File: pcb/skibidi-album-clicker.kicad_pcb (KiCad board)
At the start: 2 copper layers, 28 x 60 mm, 28 parts, among them J1 Conn_01x02_Socket, Q1 Q_PMOS_GSD, Q2 Q_NMOS_GSD, SW1 RotaryEncoder_Switch, U1 XIAO-RP2040-DIP, U2 MCP73831-2-OT

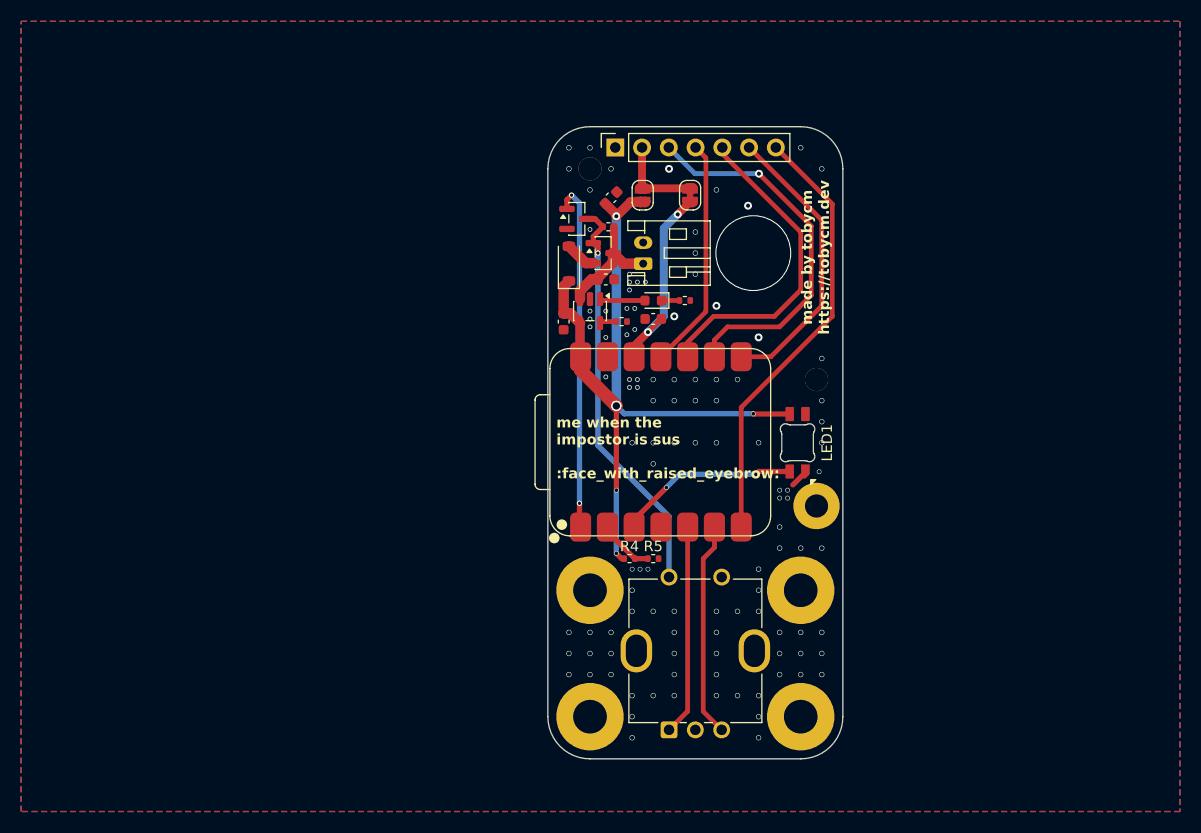
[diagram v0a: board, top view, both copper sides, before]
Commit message: update
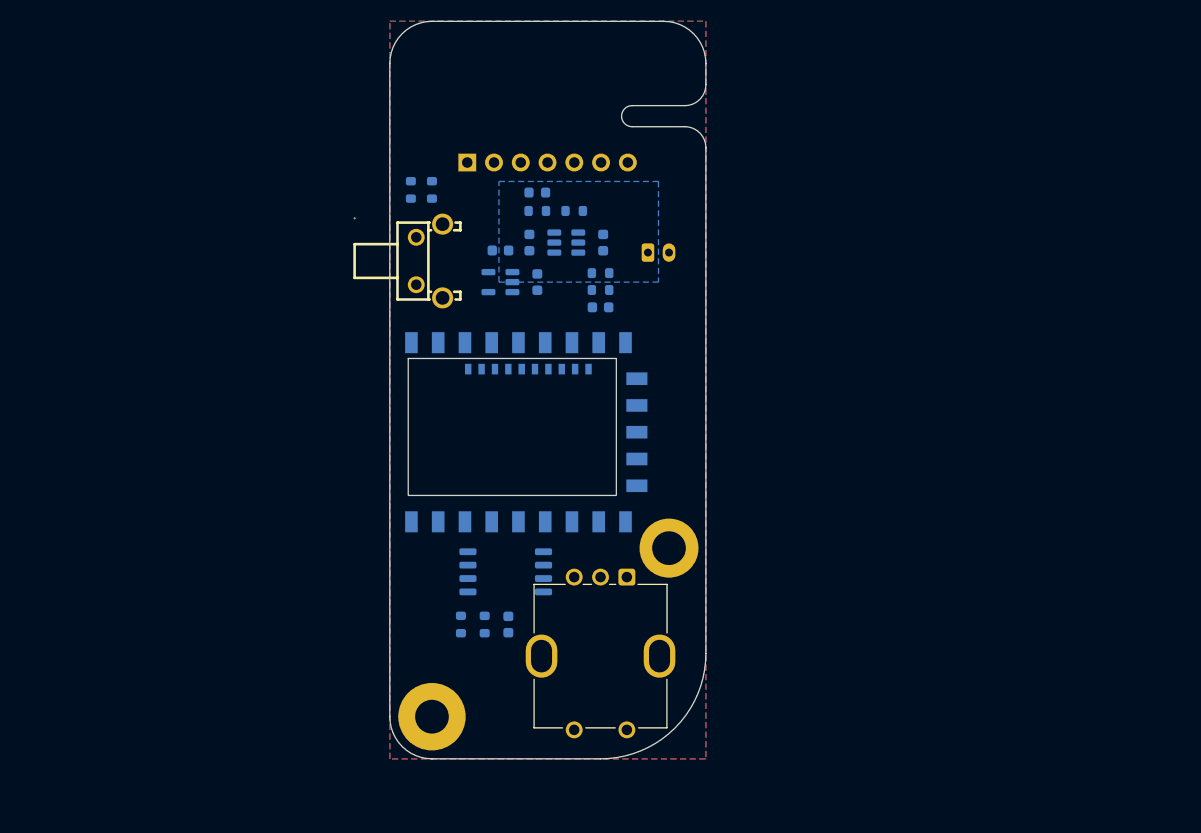
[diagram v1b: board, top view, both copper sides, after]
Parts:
- removed C2, C3: 4.7u, Capacitor_SMD:C_0603_1608Metric
- removed D2: D_Schottky, Diode_SMD:D_SOD-123
- removed H3, H4: MountingHole, MountingHole:MountingHole_3.2mm_M3_Pad
- removed H5, H7, H8: MountingHole, MountingHole:MountingHole_2.2mm_M2_Pad
- removed JP1: SolderJumper_2_Bridged, Jumper:SolderJumper-2_P1.3mm_Bridged_RoundedPad1.0x1.5mm
- removed JP2: SolderJumper_2_Open, Jumper:SolderJumper-2_P1.3mm_Open_RoundedPad1.0x1.5mm
- removed LED1: SK6812MINI-E, PCM_marbastlib-various:LED_6028R
- removed Q1: Q_PMOS_GSD, Package_TO_SOT_SMD:SOT-23
- removed Q2: Q_NMOS_GSD, Package_TO_SOT_SMD:SOT-23
- added C5: 10u, Capacitor_SMD:C_0603_1608Metric, B.Cu at (198.2, 71.0)
- added C6: 10u, Capacitor_SMD:C_0603_1608Metric, B.Cu at (205.2, 71.0)
- added C7: 10u, Capacitor_SMD:C_0603_1608Metric, B.Cu at (199.0, 74.8)
- added C8: 10u, Capacitor_SMD:C_0603_1608Metric, B.Cu at (195.5, 71.8)
- added R6: 2.49k, Resistor_SMD:R_0603_1608Metric, B.Cu at (205.0, 75.5)
- added R7: 1k, Resistor_SMD:R_0603_1608Metric, B.Cu at (202.5, 68.0)
- added R8: 2.49k, Resistor_SMD:R_0603_1608Metric, B.Cu at (199.0, 68.0)
- added SW2: K2-1102AQ-H4CW-01, easyeda2kicad:SW-TH_K2-1102BQ-G4CW-01, F.Cu at (188.8, 72.8)
- added U3: TP4057, Package_TO_SOT_SMD:TSOT-23-6, B.Cu at (201.8, 71.0)
- added U4: ME6211C33M5, Package_TO_SOT_SMD:SOT-23-5, B.Cu at (195.5, 74.8)
- C1: value 4.7u -> 10u; moved to B.Cu
- C4: value 4.7u -> 100n; moved to B.Cu
- D1, J1: moved to B.Cu
- DS1: footprint misc:IPS LCD Display -> Connector_PinSocket_2.54mm:PinSocket_1x07_P2.54mm_Horizontal; moved to B.Cu
- R1, R2: value 2k -> 2.49k; footprint Resistor_SMD:R_0402_1005Metric -> Resistor_SMD:R_0603_1608Metric; moved to B.Cu
- R3, R4, R5: value 100k -> 2.49k; footprint Resistor_SMD:R_0402_1005Metric -> Resistor_SMD:R_0603_1608Metric; moved to B.Cu
- U1: value XIAO-RP2040-DIP -> PY25Q128HA-SUH-IR; footprint Seeed Studio XIAO Series Library:XIAO-RP2040-Simple-SMD -> Package_SO:SOIC-8_5.3x5.3mm_P1.27mm; moved to B.Cu
- U2: value MCP73831-2-OT -> RP2040-ZERO; footprint Package_TO_SOT_SMD:SOT-23-5 -> easyeda2kicad:COMM-SMD_RP2040-ZERO; moved to B.Cu
- moved R4 40.7 mm to (187.0, 66.0), turned to 90 degrees
- moved R2 36.1 mm to (194.0, 107.2), turned to 90 degrees
- moved H1 35.0 mm to (189.0, 116.0)
- moved R1 32.5 mm to (191.8, 107.2), turned to 90 degrees
- moved C1 29.2 mm to (196.2, 107.2)
- moved R5 27.6 mm to (205.0, 73.9), turned to 180 degrees
- moved U1 19.2 mm to (196.0, 102.2), turned to 0 degrees
- moved H2 17.7 mm to (211.5, 100.0)
- moved R3 17.1 mm to (189.0, 66.0), turned to -90 degrees
- moved SW1 15.0 mm to (207.5, 102.8), turned to -90 degrees
- moved D1 15.0 mm to (199.0, 66.2)
- moved DS1 14.1 mm to (192.3, 63.4), turned to -90 degrees
- moved U2 13.1 mm to (197.8, 89.0)
- moved C4 5.12 mm to (205.0, 77.1), turned to 0 degrees
- moved J1 1.14 mm to (209.5, 72.0), turned to 0 degrees
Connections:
- C1 pad 1: VBUS -> +3V3
- C4 pad 1: +3.3V -> /B_VOLT
- C4 pad 2: GND -> /B_VOLT_REF
- D1 pad 2: Net-(D1-A) -> +5V
- DS1 pad 2: Net-(DS1-VCC) -> +3V3
- DS1 pad 3: Net-(DS1-SCL) -> /SCK2
- DS1 pad 4: Net-(DS1-SDA) -> /MOSI2
- R1 pad 1: Net-(U2-PROG) -> +3V3
- R1 pad 2: GND -> Net-(U1-~{WP}/IO_{2})
- R2 pad 1: Net-(D1-K) -> +3V3
- R2 pad 2: GND -> Net-(U1-~{HOLD}/~{RESET}/IO_{3})
- R3 pad 2: Net-(Q1-G) -> Net-(R3-Pad2)
- R4 pad 1: VBUS -> Net-(R3-Pad2)
- R4 pad 2: Net-(U1-GPIO27/ADC1/A1) -> GND
- R5 pad 1: Net-(U1-GPIO27/ADC1/A1) -> +BATT
- R5 pad 2: GND -> /B_VOLT
- SW1 pad A: Net-(U1-GPIO6/SDA) -> /A
- SW1 pad B: Net-(U1-GPIO7/SCL) -> /B
- SW1 pad S1: Net-(Q1-G) -> GND
- SW1 pad S2: GND -> /E_SW
- U1 pad 1: Net-(Q2-G) -> /CS
- U1 pad 2: Net-(U1-GPIO27/ADC1/A1) -> /MISO
- U1 pad 3: /Neopixel -> Net-(U1-~{WP}/IO_{2})
- U1 pad 4: unconnected-(U1-GPIO29/ADC3/A3-Pad4) -> GND
- U1 pad 5: Net-(U1-GPIO6/SDA) -> /MOSI
- U1 pad 6: Net-(U1-GPIO7/SCL) -> /SCK
- U1 pad 7: /BLK -> Net-(U1-~{HOLD}/~{RESET}/IO_{3})
- U1 pad 8: /DC -> +3V3
- U2 pad 1: Net-(D1-A) -> /MISO
- U2 pad 2: GND -> /CS
- U2 pad 3: +BATT -> /SCK
- U2 pad 4: VBUS -> /MOSI
- U2 pad 5: Net-(U2-PROG) -> /A
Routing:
- net VBUS: track 68.9 -> 0.00 mm, vias 5 -> 0
- net /BLK: track 41.8 -> 0.00 mm
- net Net-(Q1-G): track 38.5 -> 0.00 mm, vias 1 -> 0
- net Net-(DS1-SCL): track 35.7 -> 0.00 mm, vias 1 -> 0
- net Net-(Q2-G): track 33.3 -> 0.00 mm, vias 2 -> 0
- net /RES: track 30.8 -> 0.00 mm
- net /DC: track 27.5 -> 0.00 mm
- net Net-(DS1-SDA): track 22.0 -> 0.00 mm
- net Net-(U1-GPIO7/SCL): track 20.4 -> 0.00 mm
- net Net-(U1-GPIO6/SDA): track 20.0 -> 0.00 mm
- net +3.3V: track 18.7 -> 0.00 mm, vias 2 -> 0
- net /Neopixel: track 17.3 -> 0.00 mm, vias 2 -> 0
- net +BATT: track 11.8 -> 0.00 mm
- net Net-(DS1-VCC): track 8.40 -> 0.00 mm
- net Net-(U1-GPIO27/ADC1/A1): track 5.32 -> 0.00 mm
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- added copper zone on B.Cu, net +3V3
- added copper zone on B.Cu, net +BATT
- removed copper zone on B.Cu, net GND
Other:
- board size 28 x 60 mm -> 30 x 70 mm
- board text removed: "made by tobycm https://tobycm.dev"
- board text removed: "me when the impostor is sus :face_with_raised_eyebrow:"
